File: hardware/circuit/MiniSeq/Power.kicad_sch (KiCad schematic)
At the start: 9 parts, among them J1 Conn_01x10_Pin, U2 TL072, U3 TL074, U4 L7809CD2T-TR

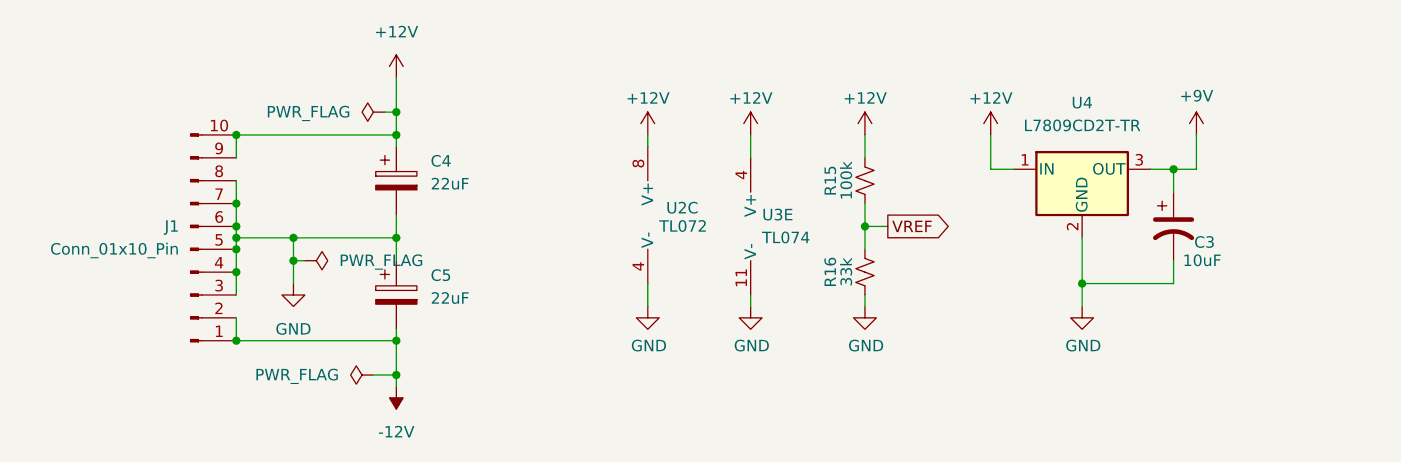
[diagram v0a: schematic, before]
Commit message: v0.1 PCBs
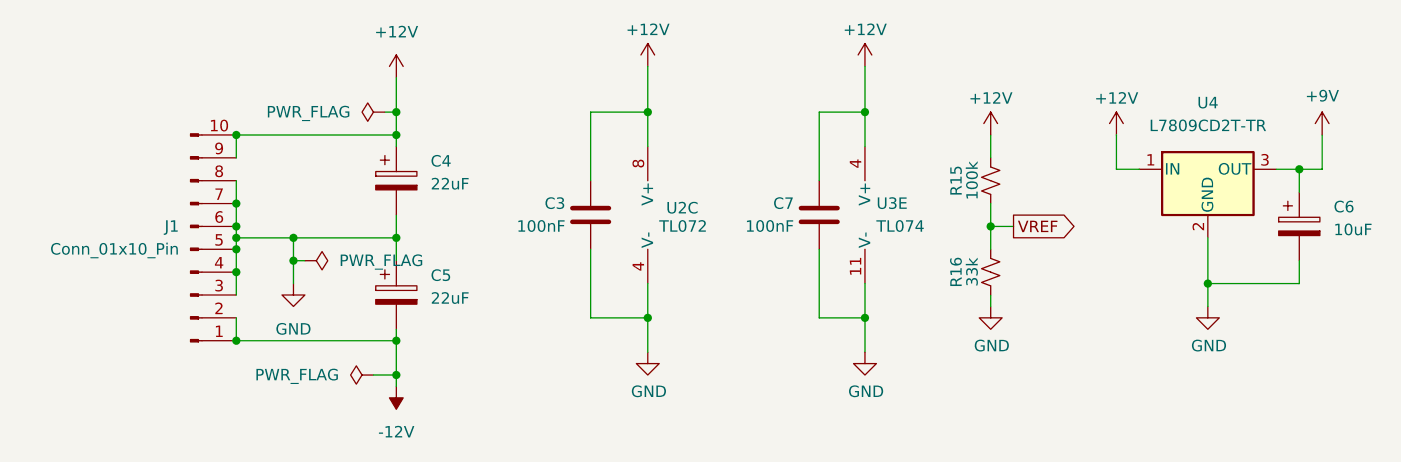
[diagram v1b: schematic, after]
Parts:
- removed C3: 10uF, Capacitor_SMD:C_0805_2012Metric_Pad1.18x1.45mm_HandSolder, symbol Device:C_Polarized_US
- added C3, C7: 100nF, Capacitor_SMD:C_0805_2012Metric_Pad1.18x1.45mm_HandSolder, symbol Device:C
- added C6: 10uF, Capacitor_SMD:CP_Elec_6.3x4.5, symbol Device:C_Polarized
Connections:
- net +12V: now also C3.1, C7.1
- net +9V: now also C6.1
- net GND: now also C3.2, C6.2, C7.2
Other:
- moved on the sheet: R15, R16, U3E, U4

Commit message: Updated PCBs for v0.1
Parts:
- C4, C5: footprint Capacitor_SMD:CP_Elec_6.3x4.5 -> Capacitor_SMD:CP_Elec_4x3.9
- C6: footprint Capacitor_SMD:CP_Elec_6.3x4.5 -> Capacitor_SMD:C_0805_2012Metric_Pad1.18x1.45mm_HandSolder
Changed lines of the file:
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@@
 			)
 		)
-		(property "Footprint" "Capacitor_SMD:CP_Elec_6.3x4.5"
+		(property "Footprint" "Capacitor_SMD:CP_Elec_4x3.9"
 			(at 74.6252 72.39 0)
 			(effects
@@
 			)
 		)
-		(property "Footprint" "Capacitor_SMD:CP_Elec_6.3x4.5"
+		(property "Footprint" "Capacitor_SMD:C_0805_2012Metric_Pad1.18x1.45mm_HandSolder"
 			(at 174.9552 64.77 0)
 			(effects
@@
 			)
 		)
-		(property "Footprint" "Capacitor_SMD:CP_Elec_6.3x4.5"
+		(property "Footprint" "Capacitor_SMD:CP_Elec_4x3.9"
 			(at 74.6252 59.69 0)
 			(effects
